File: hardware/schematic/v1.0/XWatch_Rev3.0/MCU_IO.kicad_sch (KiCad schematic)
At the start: 11 parts, among them U1 STM32U5G9NJH6Q, X1 32.768KHZ, X2 16MHZ

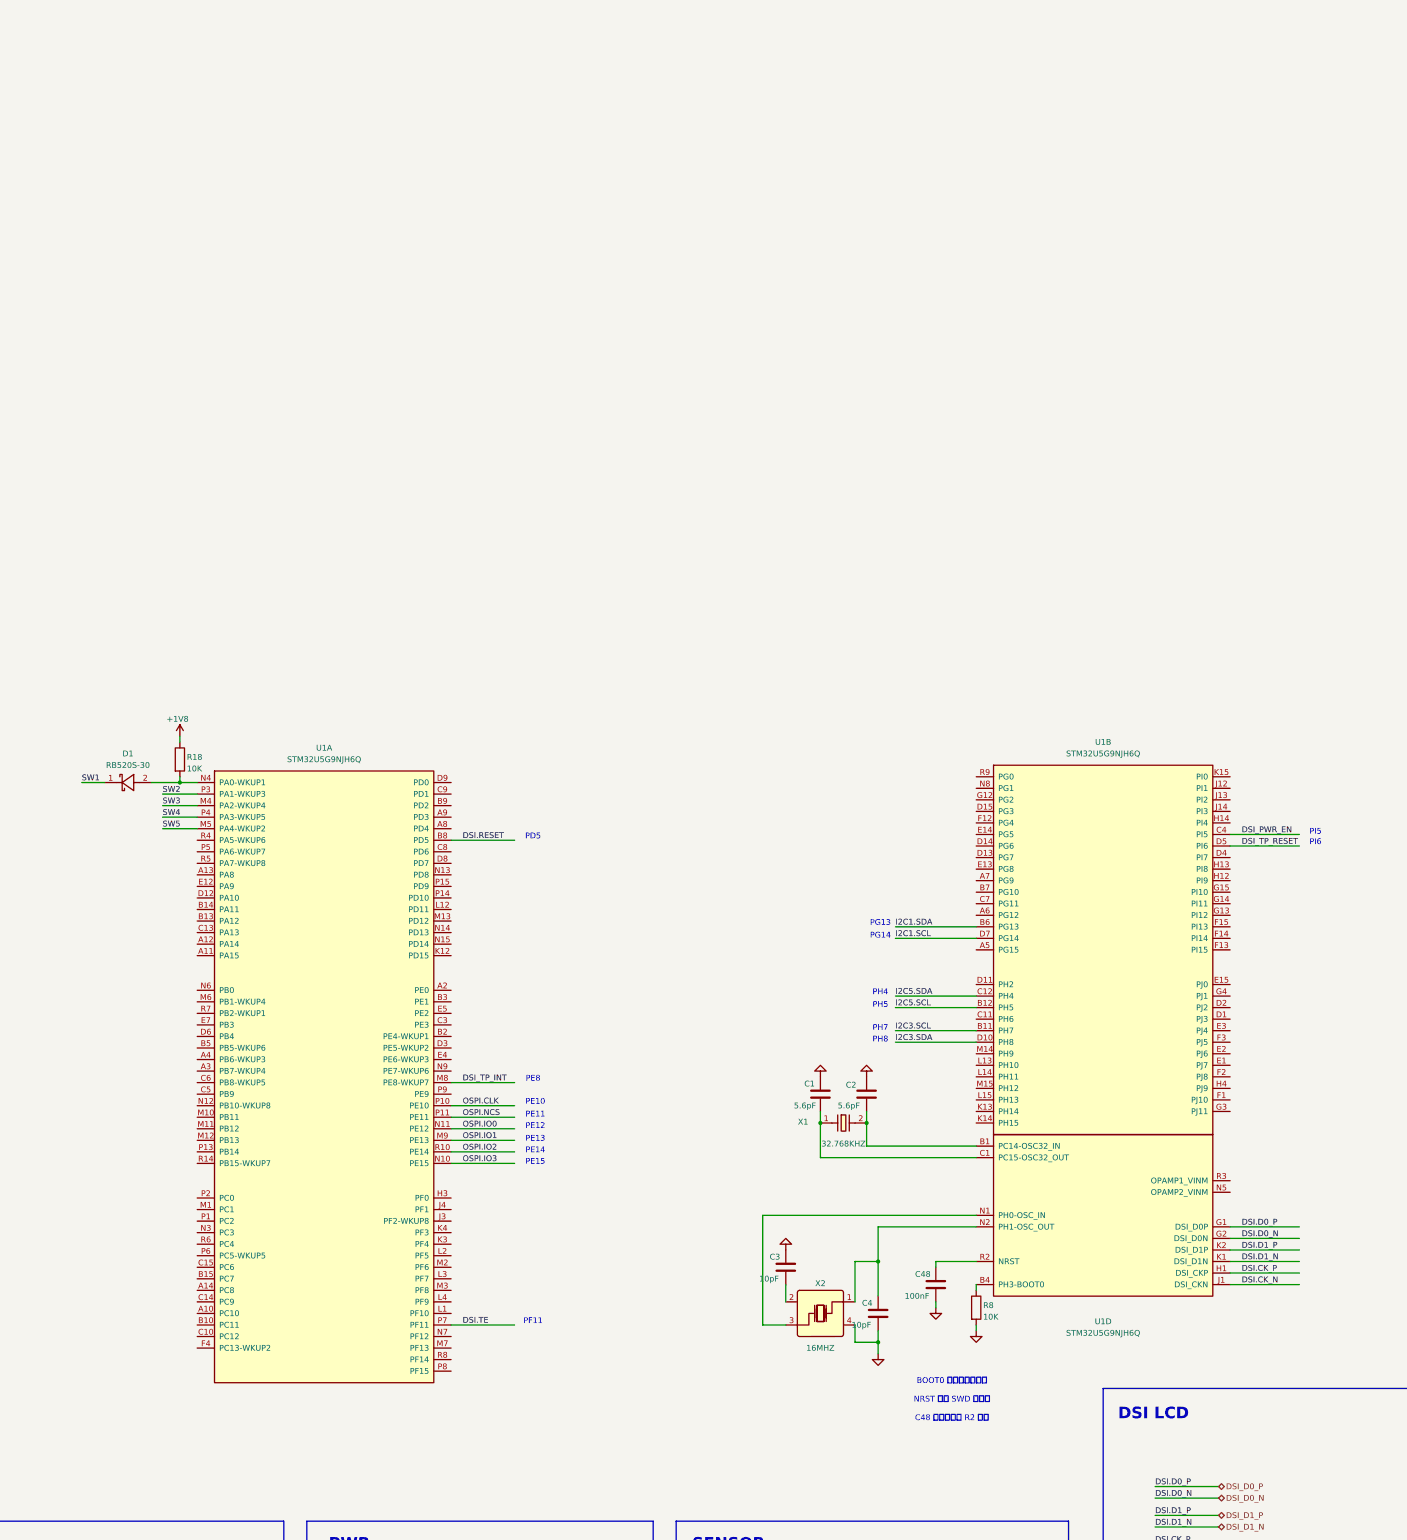
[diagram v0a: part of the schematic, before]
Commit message: sch update
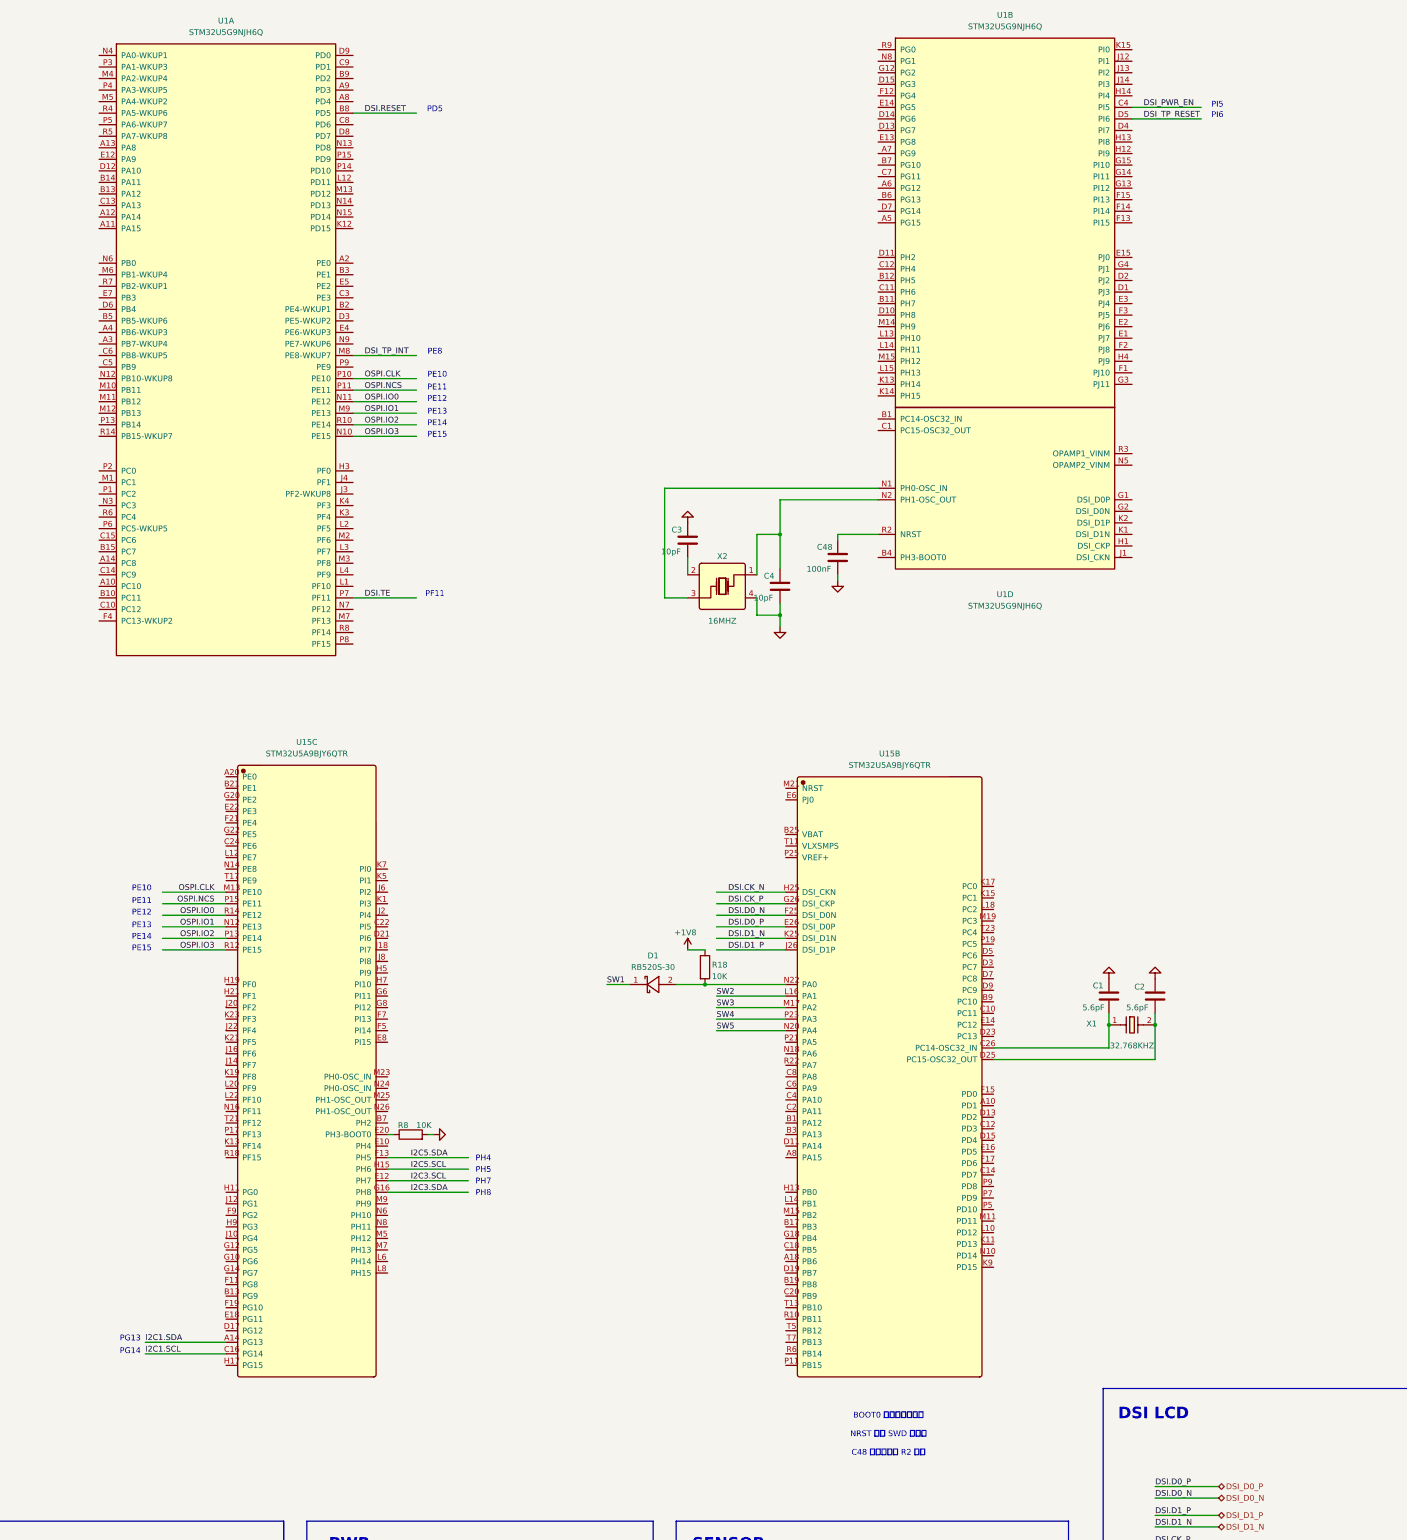
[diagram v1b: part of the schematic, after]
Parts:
- added U15: STM32U5A9BJY6QTR, XWatch_Rev3.0:STM32U5A9BJY6QTR, symbol XWatch_Rev3.0:STM32U5A9BJY6QTR
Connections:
- net DSI_CK_N: now also U15.H25 (DSI_CKN); no longer U1.J1 (DSI_CKN)
- net DSI_CK_P: now also U15.G26 (DSI_CKP); no longer U1.H1 (DSI_CKP)
- net DSI_D0_N: now also U15.F25 (DSI_D0N); no longer U1.G2 (DSI_D0N)
- net DSI_D0_P: now also U15.E26 (DSI_D0P); no longer U1.G1 (DSI_D0P)
- net DSI_D1_N: now also U15.K25 (DSI_D1N); no longer U1.K1 (DSI_D1N)
- net DSI_D1_P: now also U15.J26 (DSI_D1P); no longer U1.K2 (DSI_D1P)
- net OSPI_CLK: now also U15.M13 (PE10)
- net OSPI_IO0: now also U15.R14 (PE12)
- net OSPI_IO1: now also U15.N12 (PE13)
- net OSPI_IO2: now also U15.P13 (PE14)
- net OSPI_IO3: now also U15.R12 (PE15)
- net OSPI_NCS: now also U15.P15 (PE11)
- net PWR_SCL: now also U15.C16 (PG14); no longer U1.D7 (PG14)
- net PWR_SDA: now also U15.A14 (PG13); no longer U1.B6 (PG13)
- net SENSOR_SCL: now also U15.E12 (PH7); no longer U1.B11 (PH7)
- net SENSOR_SDA: now also U15.G16 (PH8); no longer U1.D10 (PH8)
- net SW2: now also U15.L16 (PA1); no longer U1.P3 (PA1-WKUP3)
- net SW3: now also U15.M17 (PA2); no longer U1.M4 (PA2-WKUP4)
- net SW4: now also U15.P23 (PA3); no longer U1.P4 (PA3-WKUP5)
- net SW5: now also U15.N20 (PA4); no longer U1.M5 (PA4-WKUP2)
- net TP_SCL: now also U15.H15 (PH6); no longer U1.B12 (PH5)
- net TP_SDA: now also U15.F13 (PH5); no longer U1.C12 (PH4)
- net at C2.2, X1.2: now also U15.D25 (PC15-OSC32_OUT); no longer U1.B1 (PC14-OSC32_IN)
- net at U1.B4 (PH3-BOOT0): no longer R8.1
- net at C1.2, X1.1: now also U15.C26 (PC14-OSC32_IN); no longer U1.C1 (PC15-OSC32_OUT)
- net at D1.2 (A), R18.2: now also U15.N22 (PA0); no longer U1.N4 (PA0-WKUP1)
- new net: R8.1, U15.E20 (PH3-BOOT0)
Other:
- moved on the sheet: C3, C4, C48, U1A, U1B, U1D, X2
